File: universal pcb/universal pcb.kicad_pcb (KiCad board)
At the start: 2 copper layers, 30 x 22.5 mm, 6 parts

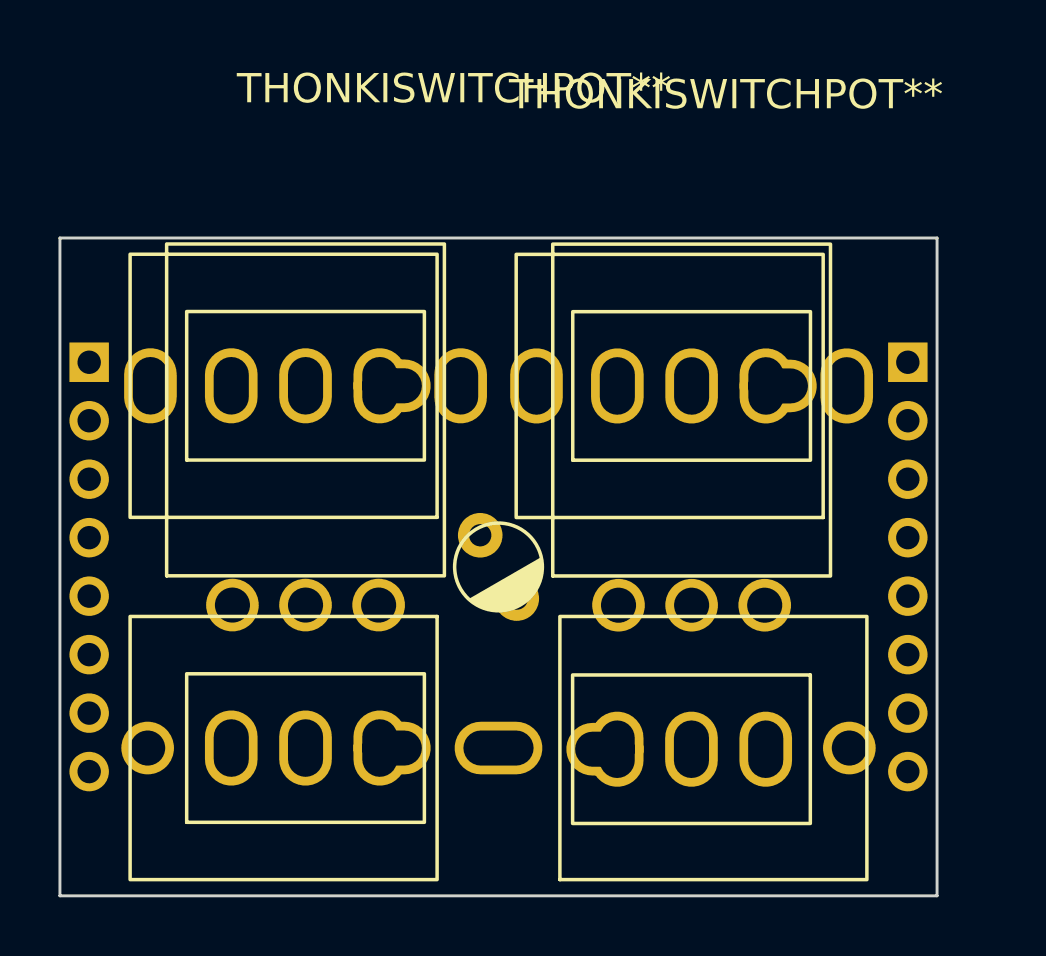
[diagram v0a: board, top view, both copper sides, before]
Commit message: KiCad Changes
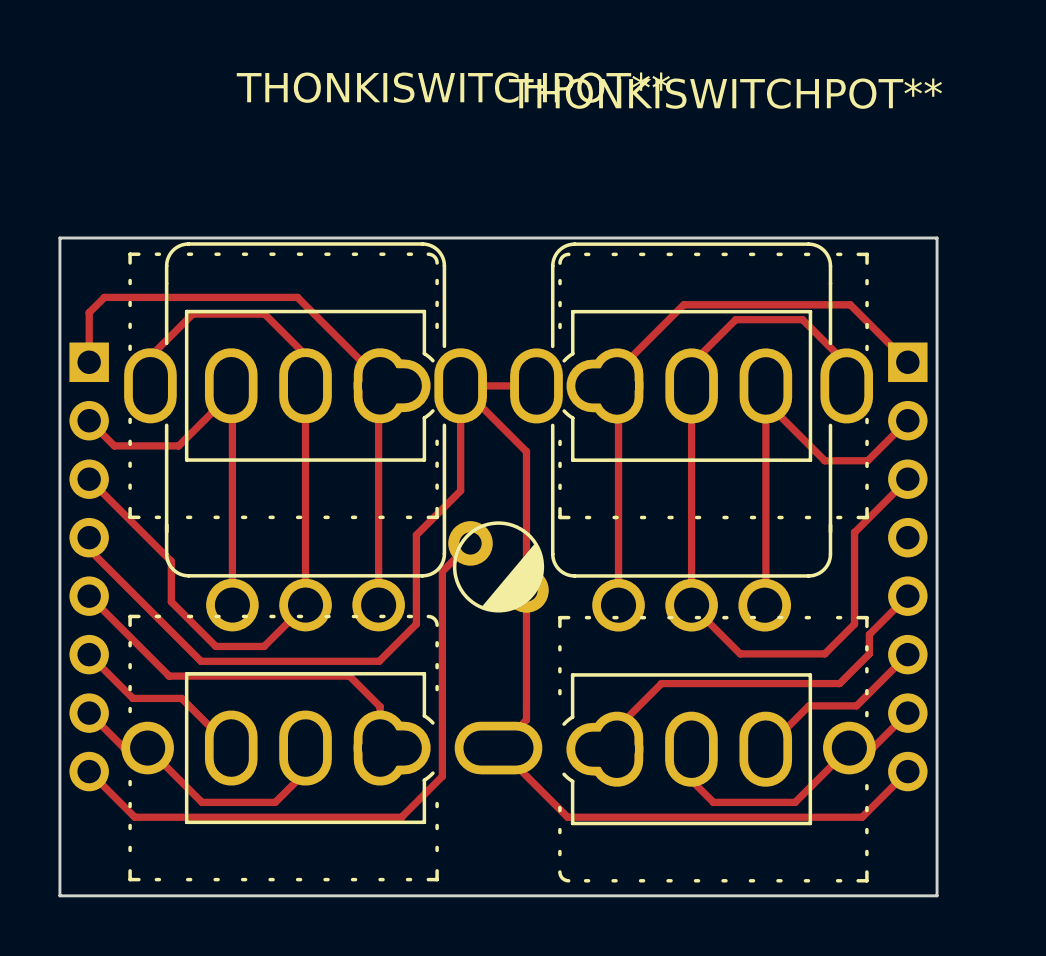
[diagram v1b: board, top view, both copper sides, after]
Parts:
- turned LED to -40 degrees
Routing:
- net (no net): track 0.00 -> 260.0 mm
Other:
- board text added: "gnd"
- board text added: "led"
- board text added: "x"
- board text added: "y"
- board text added: "z"
